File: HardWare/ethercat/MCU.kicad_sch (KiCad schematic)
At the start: 47 parts, among them J2 Conn_01x03, J3 Conn_01x04, J6 Conn_01x03, J7 Conn_01x04, SW1 SW_Push, U5 STM32F407VETx, U6 TJA1051T-3, U7 TJA1051T-3, Y1 8M, Y2 32.768KHz

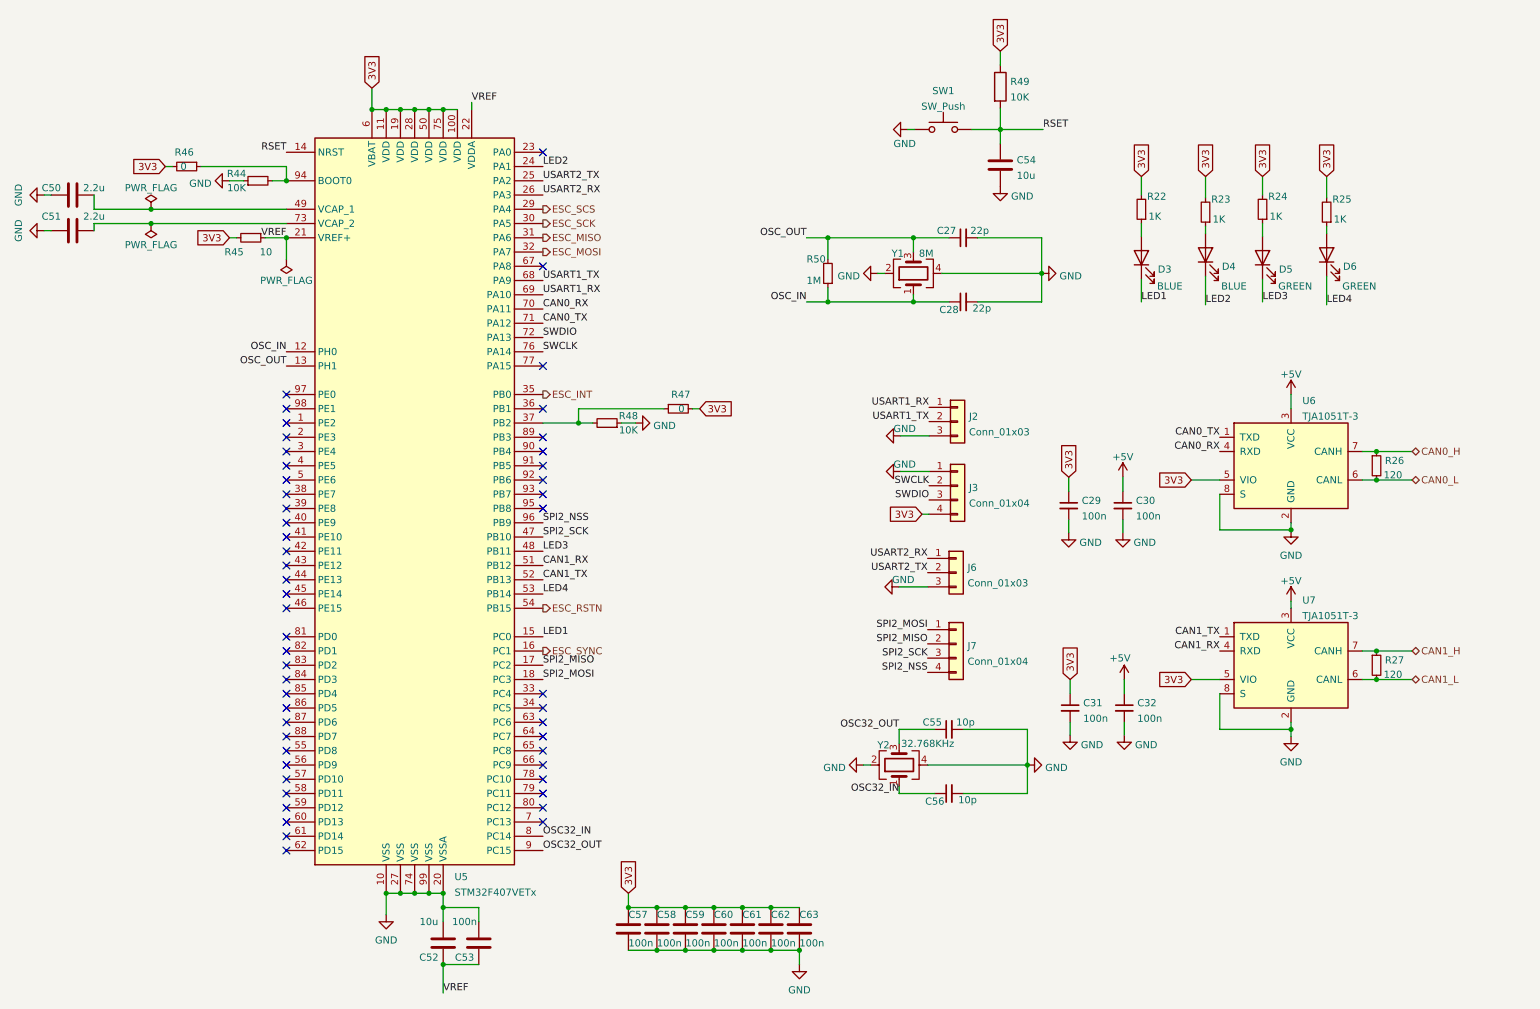
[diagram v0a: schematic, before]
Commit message: Official version-EtherCAT2CAN_NUC
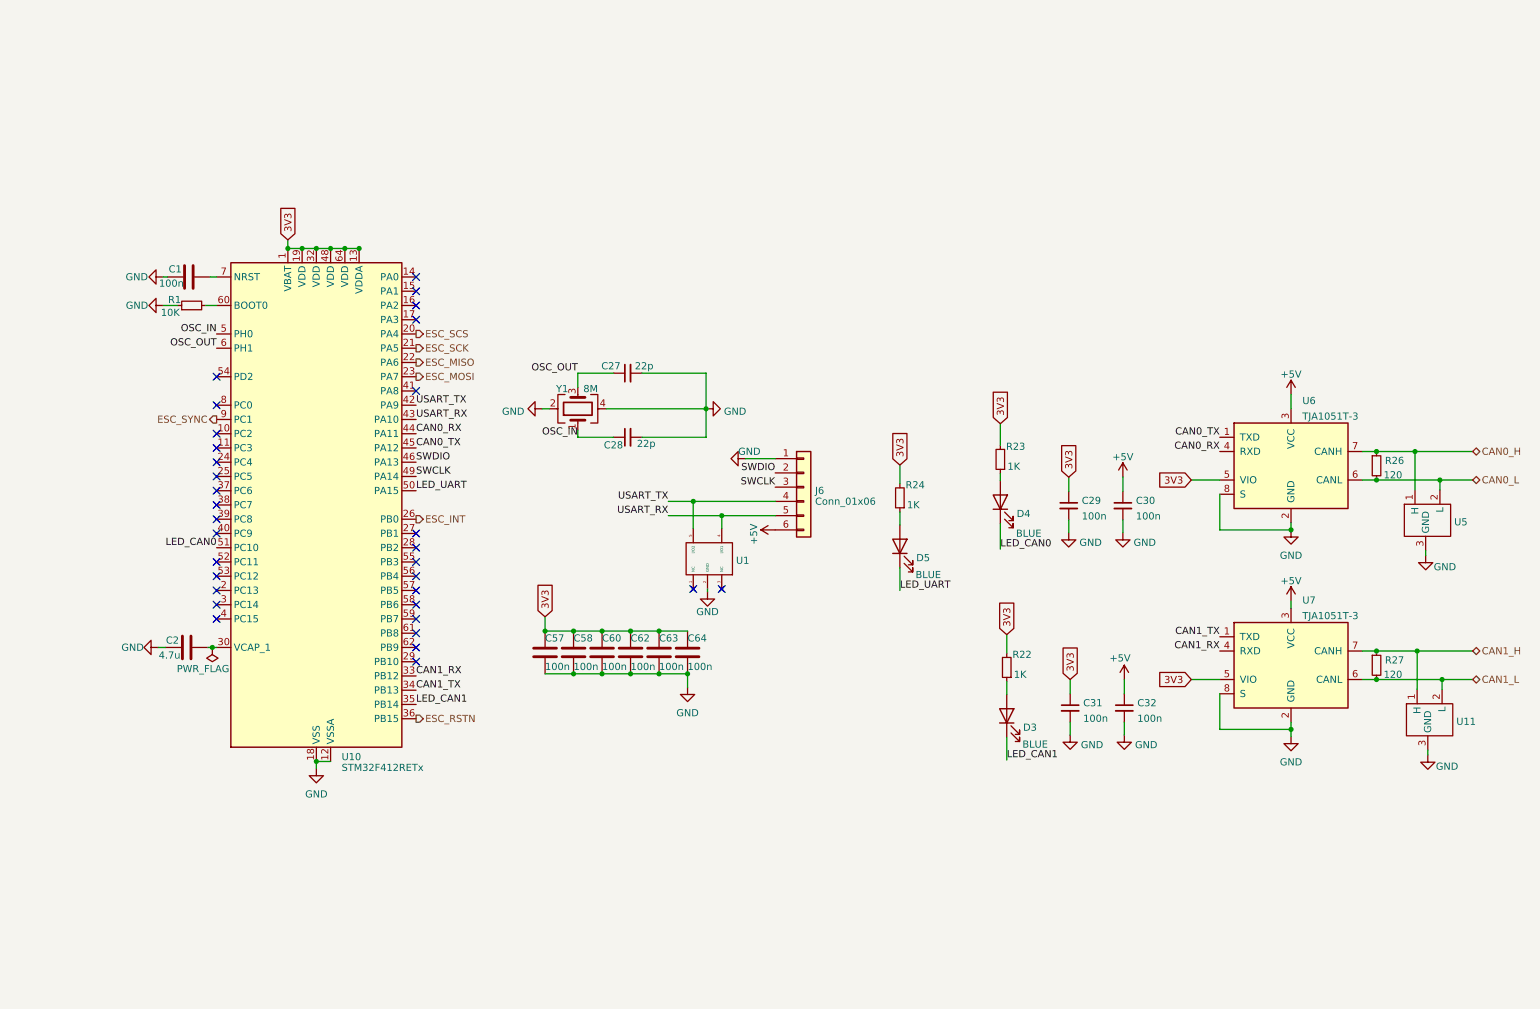
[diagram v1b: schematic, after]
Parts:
- removed C50, C51: 2.2u, Capacitor_SMD:C_0603_1608Metric, symbol Device:C
- removed C52, C54: 10u, Capacitor_SMD:C_0603_1608Metric, symbol Device:C
- removed C53, C59, C61: 100n, Capacitor_SMD:C_0603_1608Metric, symbol Device:C
- removed C55, C56: 10p, Capacitor_SMD:C_0603_1608Metric, symbol Device:C_Small
- removed D6: GREEN, LED_SMD:LED_0603_1608Metric, symbol Device:LED
- removed J2, J6: Conn_01x03, Connector_JST:JST_GH_SM03B-GHS-TB_1x03-1MP_P1.25mm_Horizontal, symbol Connector_Generic:Conn_01x03
- removed J3, J7: Conn_01x04, Connector_JST:JST_GH_SM04B-GHS-TB_1x04-1MP_P1.25mm_Horizontal, symbol Connector_Generic:Conn_01x04
- removed R25: 1K, Resistor_SMD:R_0603_1608Metric, symbol Device:R_Small
- removed R44, R48: 10K, Resistor_SMD:R_0603_1608Metric, symbol Device:R_Small
- removed R45: 10, Resistor_SMD:R_0603_1608Metric, symbol Device:R_Small
- removed R46, R47: 0, Resistor_SMD:R_0603_1608Metric, symbol Device:R_Small
- removed R49: 10K, Resistor_SMD:R_0603_1608Metric, symbol Device:R
- removed R50: 1M, Resistor_SMD:R_0603_1608Metric, symbol Device:R_Small
- removed SW1: SW_Push, Button_Switch_SMD:SW_SPST_FSMSM, symbol Switch:SW_Push
- removed U5: STM32F407VETx, Package_QFP:LQFP-100_14x14mm_P0.5mm, symbol MCU_ST_STM32F4:STM32F407VETx
- removed Y2: 32.768KHz, Crystal:Crystal_SMD_3225-4Pin_3.2x2.5mm, symbol Device:Crystal_GND24
- added C1, C64: 100n, Capacitor_SMD:C_0402_1005Metric, symbol Device:C
- added C2: 4.7u, Capacitor_SMD:C_0402_1005Metric, symbol Device:C
- added J6: Conn_01x06, Connector_JST:JST_GH_SM06B-GHS-TB_1x06-1MP_P1.25mm_Horizontal, symbol Connector_Generic:Conn_01x06
- added R1: 10K, Resistor_SMD:R_0402_1005Metric, symbol Device:R_Small
- added U1: ~, Package_TO_SOT_SMD:SOT-23-5, symbol Extra IC:ESDS314
- added U10: STM32F412RETx, Package_QFP:LQFP-64_10x10mm_P0.5mm, symbol MCU_ST_STM32F4:STM32F412RETx
- added U11, U5: ~, Package_TO_SOT_SMD:SOT-23-3, symbol Extra IC:PESD1CAN
- C27, C28, C29, C30, C31, C32, C57, C58, C60, C62, C63: footprint Capacitor_SMD:C_0603_1608Metric -> Capacitor_SMD:C_0402_1005Metric
- D3, D4: footprint LED_SMD:LED_0603_1608Metric -> LED_SMD:LED_0402_1005Metric
- D5: value GREEN -> BLUE; footprint LED_SMD:LED_0603_1608Metric -> LED_SMD:LED_0402_1005Metric
- R22, R23, R24, R26, R27: footprint Resistor_SMD:R_0603_1608Metric -> Resistor_SMD:R_0402_1005Metric
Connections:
- net +5V: now also J6.6 (Pin_6)
- net 3V3: now also C64.1, U10.1 (VBAT), U10.13 (VDDA), U10.19 (VDD), U10.32 (VDD), U10.48 (VDD), U10.64 (VDD)
- net CAN0_H: now also U5.1 (H)
- net CAN0_L: now also U5.2 (L)
- net CAN0_RX: now also U10.44 (PA11)
- net CAN0_TX: now also U10.45 (PA12)
- net CAN1_H: now also U11.1 (H)
- net CAN1_L: now also U11.2 (L)
- net CAN1_RX: now also U10.33 (PB12)
- net CAN1_TX: now also U10.34 (PB13)
- net ESC_INT: now also U10.26 (PB0)
- net ESC_MISO: now also U10.22 (PA6)
- net ESC_MOSI: now also U10.23 (PA7)
- net ESC_RSTN: now also U10.36 (PB15)
- net ESC_SCK: now also U10.21 (PA5)
- net ESC_SCS: now also U10.20 (PA4)
- net ESC_SYNC: now also U10.9 (PC1)
- net GND: now also C1.1, C2.1, C64.2, J6.1 (Pin_1), R1.1, U1.2 (GND), U10.12 (VSSA), U10.18 (VSS), U10.31 (VSS), U10.47 (VSS), U10.63 (VSS), U11.3 (GND), U5.3 (GND)
- net OSC_IN: now also U10.5 (PH0)
- net OSC_OUT: now also U10.6 (PH1)
- net SWCLK: now also J6.3 (Pin_3), U10.49 (PA14)
- net SWDIO: now also J6.2 (Pin_2), U10.46 (PA13)
- net LED1 renamed LED_CAN1
- net LED_CAN1: now also U10.35 (PB14)
- net LED2 renamed LED_CAN0
- net LED_CAN0: now also U10.51 (PC10)
- net LED3 renamed LED_UART
- net LED_UART: now also U10.50 (PA15)
- new net: C2.2, U10.30 (VCAP_1)
- new net: R1.2, U10.60 (BOOT0)
- new net: C1.2, U10.7 (NRST)
- new net USART_RX: J6.5 (Pin_5), U1.4 (I/O1), U10.43 (PA10)
- new net USART_TX: J6.4 (Pin_4), U1.5 (I/O2), U10.42 (PA9)
- no-connect marks 52 -> 32
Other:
- moved on the sheet: C27, C28, D3, D4, D5, R22, R23, R24, Y1
